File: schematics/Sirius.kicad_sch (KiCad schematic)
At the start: 10 parts, among them J1 DE9_Plug, U1 W65C02SxP, U2 W65C51NxPL, U3 6526, U4 MAX232, U5 74LS138, U6 27C64, U7 CY62256-70PC, U8 7404, X1 GTXO-14T

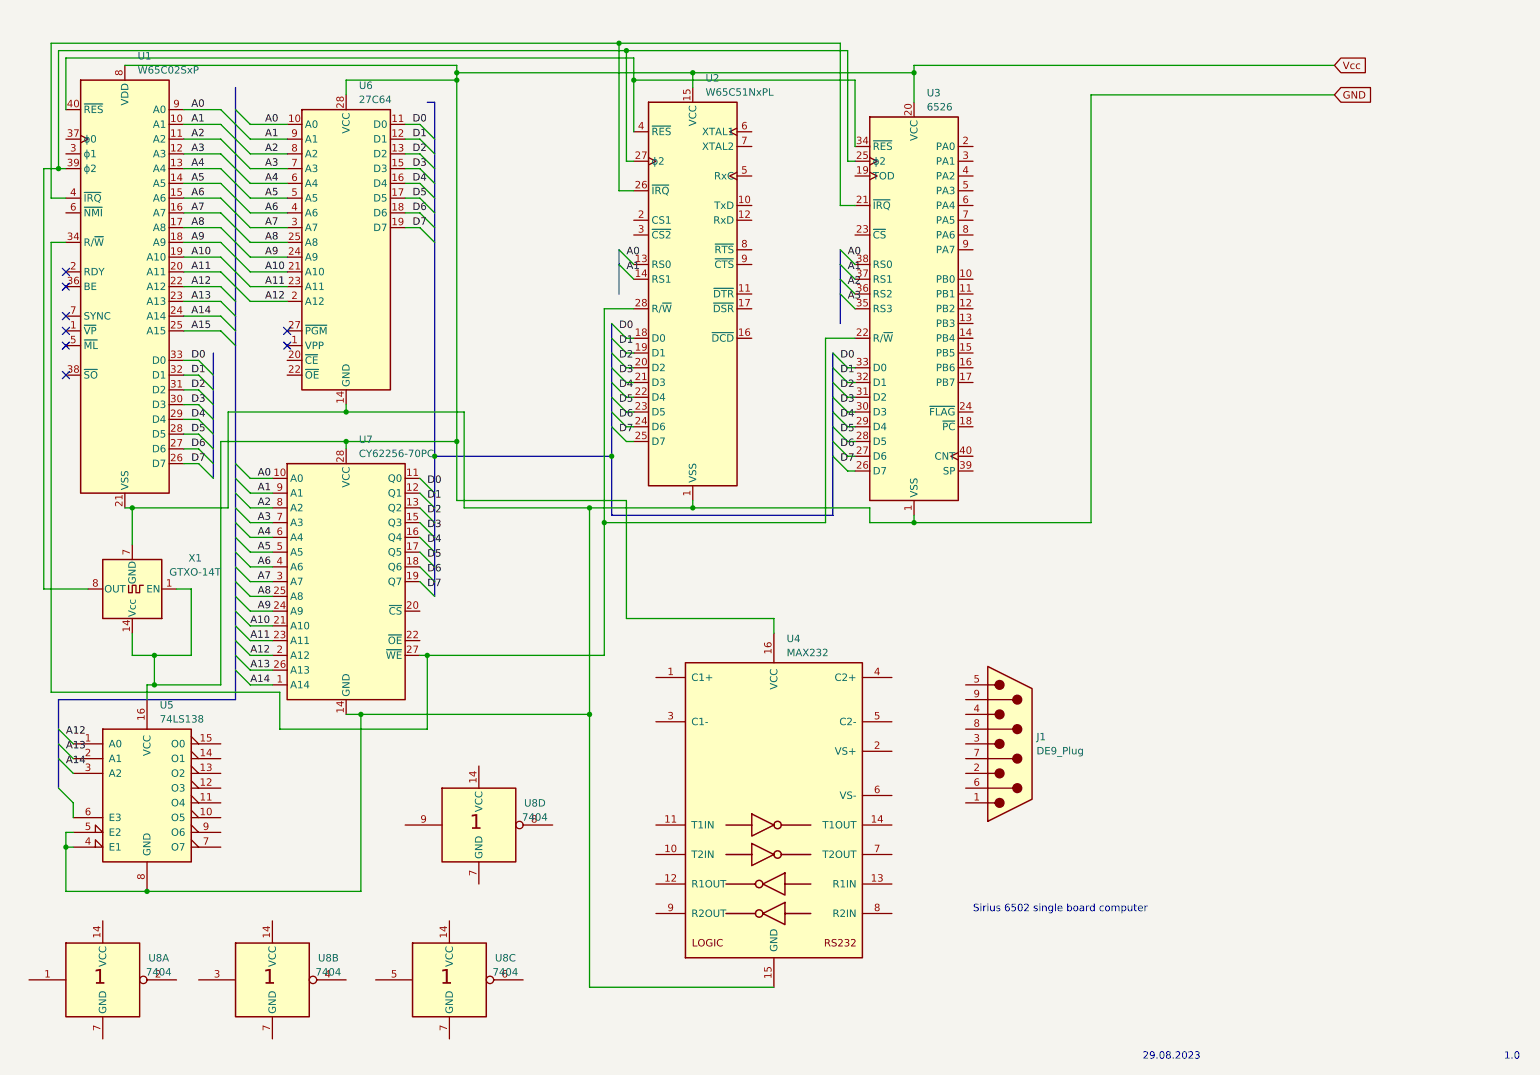
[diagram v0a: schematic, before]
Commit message: Re-worked schematics. Still lot of work to be done.
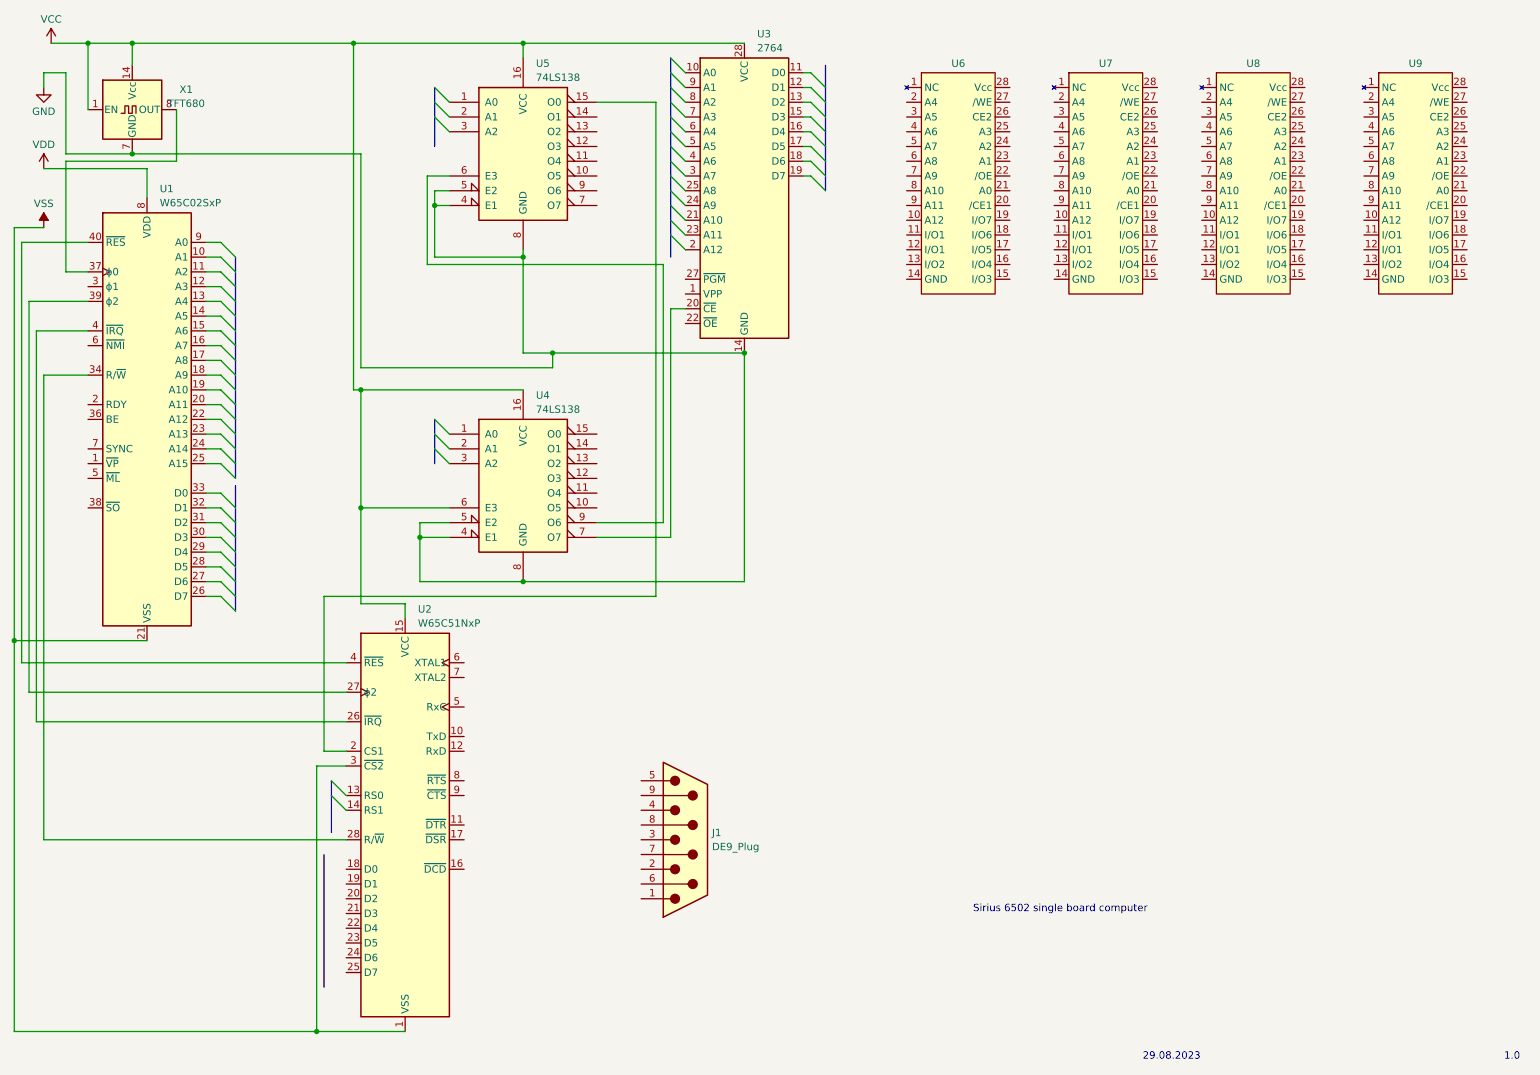
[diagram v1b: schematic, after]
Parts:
- removed U2: W65C51NxPL, Package_LCC:PLCC-28, symbol PCM_65xx-library:W65C51NxPL
- removed U3: 6526, Package_DIP:DIP-40_W15.24mm, symbol PCM_65xx-library:6526
- removed U4: MAX232, symbol Interface_UART:MAX232
- removed U6: 27C64, Package_DIP:DIP-28_W15.24mm, symbol Memory_EPROM:27C64
- removed U7: CY62256-70PC, Package_DIP:DIP-28_W15.24mm, symbol Memory_RAM:CY62256-70PC
- removed U8: 7404, symbol 74xx_IEEE:7404
- removed X1: GTXO-14T, Oscillator:Oscillator_DIP-14, symbol Oscillator:GTXO-14T
- added U2: W65C51NxP, Package_DIP:DIP-28_W15.24mm, symbol PCM_65xx-library:W65C51NxP
- added U3: 2764, Package_DIP:DIP-28_W15.24mm, symbol Memory_EPROM:2764
- added U4: 74LS138, symbol 74xx:74LS138
- added U6, U7, U8, U9: ~, symbol custom_parts:CY6264
- added X1: TFT680, Oscillator:Oscillator_DIP-14, symbol Oscillator:TFT680
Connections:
- net GND: now also U3.14 (GND), U4.4 (E1), U4.5 (E2), U4.8 (GND), X1.7 (GND); no longer U1.21 (VSS)
- net at U1.4 (~{IRQ}): now also U2.26 (~{IRQ})
- net at U1.34 (R/~{W}): now also U2.28 (R/~{W})
- net at U1.39 (ϕ2): now also U2.27 (ϕ2)
- net at U1.40 (~{RES}): now also U2.4 (~{RES})
- net at U5.15 (O0): now also U2.2 (CS1)
- net at U5.6 (E3): now also U4.9 (O6)
- net at U1.37 (ϕ0): now also X1.8 (OUT)
- net A0: no longer names the net of U1.9 (A0)
- net A1: no longer names the net of U1.10 (A1)
- net A10: no longer names the net of U1.19 (A10)
- net A11: no longer names the net of U1.20 (A11)
- net A12: no longer names the net of U1.22 (A12)
- net A13: no longer names the net of U1.23 (A13)
- net A14: no longer names the net of U1.24 (A14)
- net A15: no longer names the net of U1.25 (A15)
- net A2: no longer names the net of U1.11 (A2)
- net A3: no longer names the net of U1.12 (A3)
- net A4: no longer names the net of U1.13 (A4)
- net A5: no longer names the net of U1.14 (A5)
- net A6: no longer names the net of U1.15 (A6)
- net A7: no longer names the net of U1.16 (A7)
- net A8: no longer names the net of U1.17 (A8)
- net A9: no longer names the net of U1.18 (A9)
- net D0: no longer names the net of U1.33 (D0)
- net D1: no longer names the net of U1.32 (D1)
- net D2: no longer names the net of U1.31 (D2)
- net D3: no longer names the net of U1.30 (D3)
- net D4: no longer names the net of U1.29 (D4)
- net D5: no longer names the net of U1.28 (D5)
- net D6: no longer names the net of U1.27 (D6)
- net D7: no longer names the net of U1.26 (D7)
- net Vcc renamed VCC
- net VCC: now also U2.15 (VCC), U3.28 (VCC), U4.16 (VCC), U4.6 (E3), X1.1 (EN), X1.14 (Vcc); no longer U1.8 (VDD)
- new net: U3.20 (~{CE}), U4.7 (O7)
- new net VDD: U1.8 (VDD)
- new net VSS: U1.21 (VSS), U2.1 (VSS), U2.3 (~{CS2})
- no-connect marks 8 -> 0
